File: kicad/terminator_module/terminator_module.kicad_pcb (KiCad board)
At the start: 2 copper layers, 36 x 16 mm, 8 parts, among them J1 Coax, J2 Coax

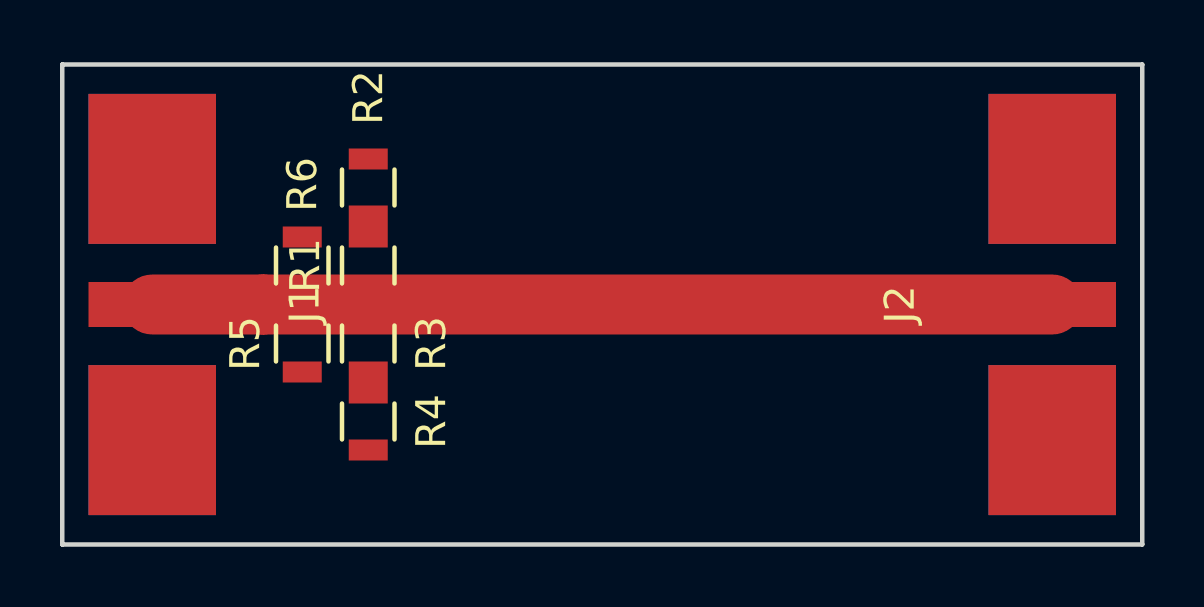
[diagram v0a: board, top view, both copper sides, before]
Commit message: * small mods
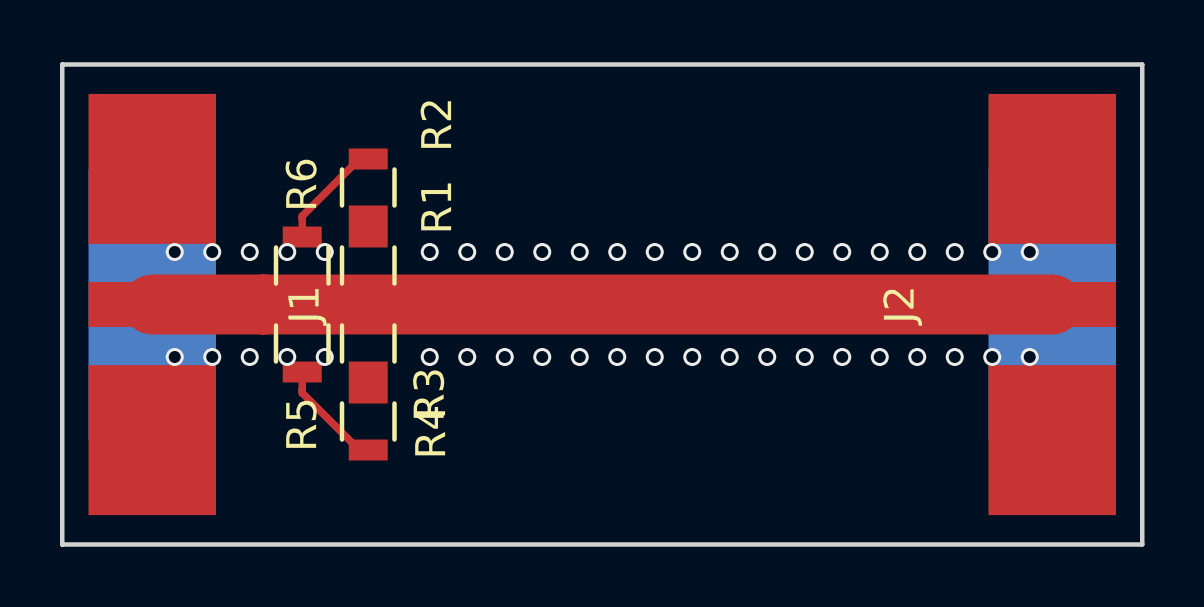
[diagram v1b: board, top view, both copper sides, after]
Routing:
- net GND: track 0.00 -> 7.37 mm, vias 0 -> 44
- net Net-(R3-Pad2): track 0.00 -> 0.70 mm
- net Net-(R1-Pad2): track 0.00 -> 0.70 mm
- net Net-(J1-Pad2): track 47.7 -> 48.4 mm
- added copper zone on B.Cu, net GND
